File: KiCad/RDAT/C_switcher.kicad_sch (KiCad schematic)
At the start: 11 parts, among them J18 MUSBRM1C130, U10 CH224K

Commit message: Push before Board Layout
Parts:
- C78: footprint A_HDJ_Library:C_0402_1005Metric -> Capacitor_SMD:C_0402_1005Metric
- D126, D127, D128: footprint A_HDJ_Library:D_0402_1005Metric -> Diode_SMD:D_SOD-882
- J18: footprint A_HDJ_Library:USB_C_Receptacle_G-Switch_GT-USB-7010ASV -> footprints:AMPHENOL_MUSBRM1C130
- R69, R70, R71: footprint A_HDJ_Library:R_0402_1005Metric -> Resistor_SMD:R_0402_1005Metric
- U10: footprint A_HDJ_Library:ESSOP-10-1EP_3.9x5mm_P1.0mm_EP3.2x2.3 -> footprints:ESSOP-10_L4.9-W3.9-P1.0-LS6.0-TL-EP
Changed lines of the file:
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@@
+			"AAAAAAAAAAAAAAAAAAAAAAAAAAAAAAAAAAAAAAAAAAAAAAAAAAAAAAAAAAAAAAAAAAAAAAAAAAAA"
+			"AAAAAAAAAAAAAAAAAAAAAAAAAAAAAAAAAAAAAAAAAAAAAAAAAAAAAAAAAAAAAAAAAAAAAAAAAAAA"
+			"AAAAAAAAAAAAAAAAAAAAAAAAAAAAAAAAAAAAAAAAAAAAAAAAAAAAAAAAAAAAAAAAAAAAAAAAAAAA"
+			"AAAAAAAAAAAAAAAAAAAAAAAAAAAAAAAAAAAAAAAAAAAAAAAAAAAAAAAAAAAAAAAAAAAAAAAAAAAA"
+			"AAAAAAAAAAAAAAAAAAAAAAAAAAAAAAAAAAAAAAAAAAAAAAAAAAAAAAAAAAAAAAAAAAAAAAAAAAAA"
+			"AAAAAAAAAAAAAAAAAAAAAAAAAAAAAAAAAAAAAAAAAAAAAAAAAAAAAAAAAAAAAAAAAAAAAAAAAAAA"
+			"AAAAAAAAAAAAAAAAAAAAAAAAAAAAAAAAAAAAAAAAAAAAAAAAAAAAAAAAAAAAAAAAAAAAAAAAAAAA"
+			"AAAAAAAAAAAAAAAAAAAAAAAAAAAAAAAAAAAAAAAAAAAAAAAAAAAAAAAAAAAAAAAAAAAAAAAAAAAA"
+			"AAAAAAAAAAAAAAAAAAAAAAAAAAAAAAAAAAAAAAAAAAAAAAAAAAAAAAAAAAAAAAAAAAAAAAAAAAAA"
+			"AAAAAAAAAAAAAAAAAAAAAAAAAAAAAAAAAAAAAAAAAAAAAAAAAAAAAAAAAAAAAAAAAAAAAAAAAAAA"
+			"AAAAAAAAAAAAAAAAAAAAAAAAAAAAAAAAAAAAAAAAAAAAAAAAAAAAAAAAAAAAAAAAAAAAAAAAAAAA"
+			"AAAAAAAAAAAAAAAAAAAAAAAAAAAAAAAAAAAAAAAAAAAAAAAAAAAAAAAAAAAAAAAAAAAAAAAAAAAA"
+			"AAAAAAAAAAAAAAAAAAAAAAAAAAAAAAAAAAAAAAAAAAAAAAAAAAAAAAAAAAAAAAAAAAAAAAAAAAAA"
+			"AAAAAAAAAAAAAAAAAAAAAAAAAAAAAAAAAAAAAAAAAAAAAAAAAAAAAAAAAAAAAAAAAAAAAAAAAAAA"
+			"AAAAAAAAAAAAAAAAAAAAAAAAAAAAAAAAAAAAAAAAAAAAAAAAAAAAAAAAAAAAAAAAAAAAAAAAAAAA"
+			"AAAAAAAAAAAAAAAAAAAAAAAAAAAAAAAAAAAAAAAAAAAAAAAAAAAAAAAAAAAAAAAAAAAAAAAAAAAA"
+			"AAAAAAAAAAAAAAAAAAAAAAAAAAAAAAAAAAAAAAAAAAAAAAAAAAAAAAAAAAAAAAAAAAAAAAAAAAAA"
+			"AAAAAAAAAAAAAAAAAAAAAAAAAAAAAAAAAAAAAAAAAAAAAAAAAAAAAAAAAAAAAAAAAAAAAAAAAAAA"
 			"AAAAAAAAAAAAAAAAAAAAAAAAAAAAAAAAAAAAAAAAAAAAAAAAAAAAAAAAAAAAAAAAAAAAAAAAAAAA"
 			"AAAAAAAAAAAAAAAAAAAAAAAAAAAAAAAAAAAAAAAAAAAAAAAAAAAAAAAAAAAAAAAAAAAAAAAAAAAA"
@@
 			)
 		)
-		(property "Footprint" "A_HDJ_Library:USB_C_Receptacle_G-Switch_GT-USB-7010ASV"
+		(property "Footprint" "footprints:AMPHENOL_MUSBRM1C130"
 			(at 60.96 53.34 0)
 			(effects
@@
 			)
 		)
-		(property "Footprint" "A_HDJ_Library:ESSOP-10-1EP_3.9x5mm_P1.0mm_EP3.2x2.3"
+		(property "Footprint" "footprints:ESSOP-10_L4.9-W3.9-P1.0-LS6.0-TL-EP"
 			(at 149.86 48.26 0)
 			(effects
@@
 			)
 		)
-		(property "Footprint" "A_HDJ_Library:D_0402_1005Metric"
+		(property "Footprint" "Diode_SMD:D_SOD-882"
 			(at 109.22 66.04 0)
 			(effects
@@
 			)
 		)
-		(property "Footprint" "A_HDJ_Library:C_0402_1005Metric"
+		(property "Footprint" "Capacitor_SMD:C_0402_1005Metric"
 			(at 127 46.6852 0)
 			(effects
@@
 			)
 		)
-		(property "Footprint" "A_HDJ_Library:D_0402_1005Metric"
+		(property "Footprint" "Diode_SMD:D_SOD-882"
 			(at 116.84 66.04 0)
 			(effects
@@
 			)
 		)
-		(property "Footprint" "A_HDJ_Library:R_0402_1005Metric"
+		(property "Footprint" "Resistor_SMD:R_0402_1005Metric"
 			(at 129.794 37.084 90)
 			(effects
@@
 			)
 		)
-		(property "Footprint" "A_HDJ_Library:D_0402_1005Metric"
+		(property "Footprint" "Diode_SMD:D_SOD-882"
 			(at 101.6 66.04 0)
 			(effects
@@
 			)
 		)
-		(property "Footprint" "A_HDJ_Library:R_0402_1005Metric"
+		(property "Footprint" "Resistor_SMD:R_0402_1005Metric"
 			(at 174.244 42.164 90)
 			(effects
@@
 			)
 		)
-		(property "Footprint" "A_HDJ_Library:R_0402_1005Metric"
+		(property "Footprint" "Resistor_SMD:R_0402_1005Metric"
 			(at 129.794 40.894 90)
 			(effects

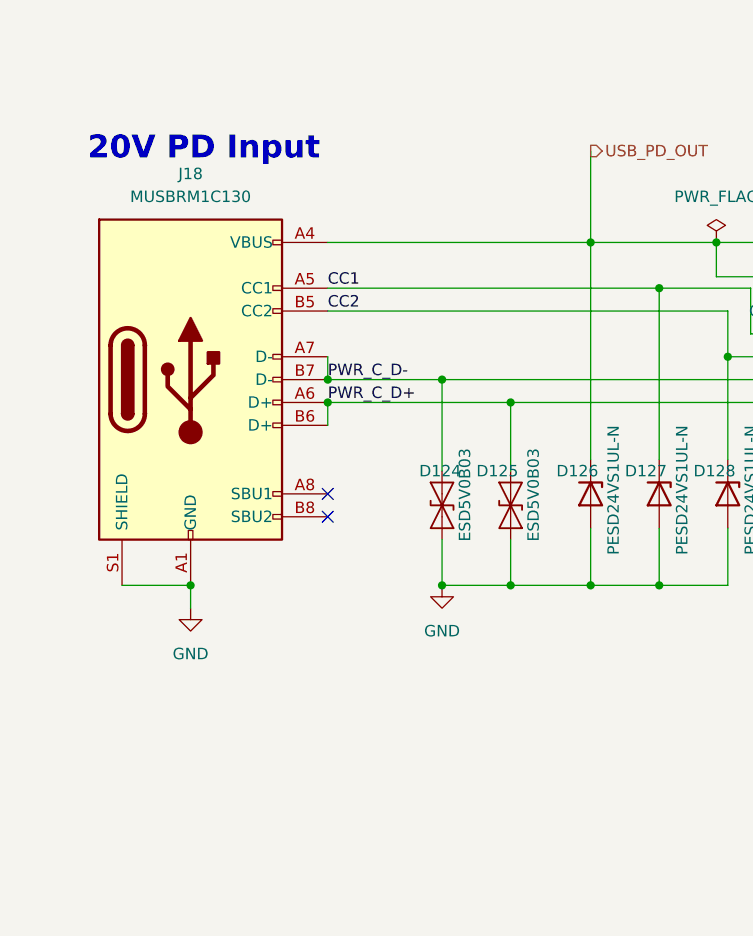
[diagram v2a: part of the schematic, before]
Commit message: Placed a lot of components
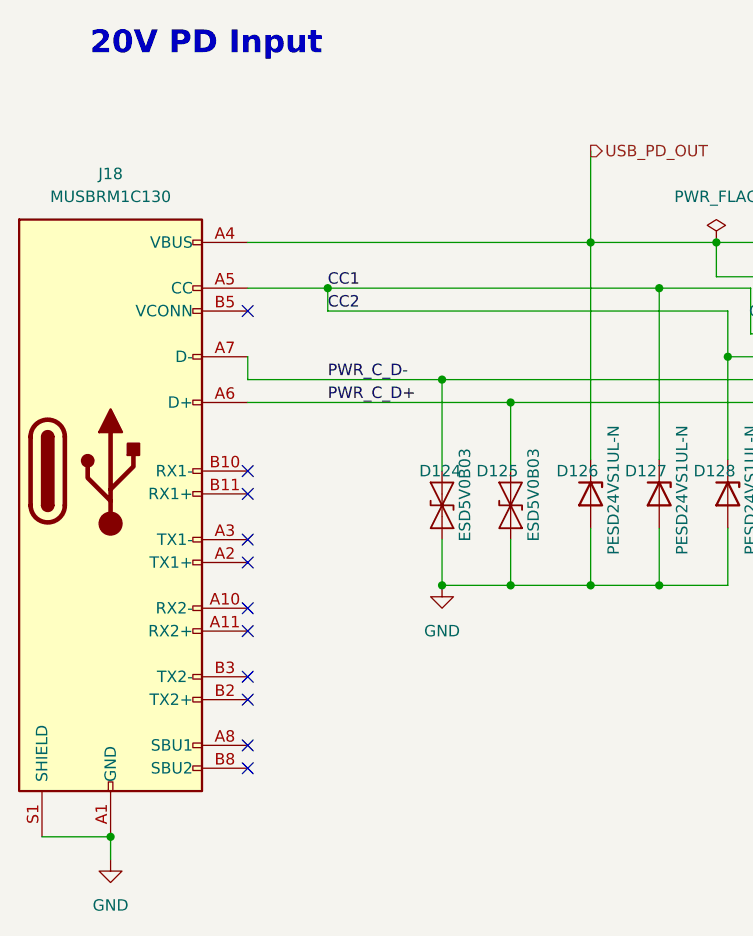
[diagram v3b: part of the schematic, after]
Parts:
- J18: symbol Connector:USB_C_Receptacle_USB2.0_16P -> Connector:USB_C_Plug
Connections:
- net CC1: now also D128.1 (K), U10.6 (CC2)
- net PWR_C_D+: no longer J18.B6 (D+)
- net PWR_C_D-: no longer J18.B7 (D-)
- removed net CC2: D128.1 (K), J18.B5 (CC2), U10.6 (CC2)
- no-connect marks 5 -> 14
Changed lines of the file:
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@@
 	(text "20V PD Input"
 		(exclude_from_sim no)
-		(at 45.72 29.21 0)
+		(at 45.974 17.526 0)
 		(effects
 			(font
@@
 	)
 	(junction
-		(at 72.39 53.34)
+		(at 72.39 43.18)
 		(diameter 0)
 		(color 0 0 0 0)
@@
 	)
 	(junction
-		(at 57.15 76.2)
-		(diameter 0)
-		(color 0 0 0 0)
-	)
-	(junction
-		(at 72.39 55.88)
-		(diameter 0)
-		(color 0 0 0 0)
-	)
-	(junction
 		(at 115.57 38.1)
 		(diameter 0)
@@
 		(color 0 0 0 0)
 	)
+	(junction
+		(at 48.26 104.14)
+		(diameter 0)
+		(color 0 0 0 0)
+	)
 	(no_connect
 		(at 162.56 45.72)
@@
 	)
 	(no_connect
-		(at 72.39 68.58)
+		(at 63.5 96.52)
 	)
 	(no_connect
-		(at 72.39 66.04)
+		(at 63.5 86.36)
+	)
+	(no_connect
+		(at 63.5 93.98)
+	)
+	(no_connect
+		(at 63.5 66.04)
+	)
+	(no_connect
+		(at 63.5 88.9)
+	)
+	(no_connect
+		(at 63.5 81.28)
 	)
 	(no_connect
 		(at 162.56 50.8)
 	)
+	(no_connect
+		(at 63.5 71.12)
+	)
+	(no_connect
+		(at 63.5 63.5)
+	)
+	(no_connect
+		(at 63.5 73.66)
+	)
+	(no_connect
+		(at 63.5 45.72)
+	)
+	(no_connect
+		(at 63.5 78.74)
+	)
 	(wire
 		(pts
@@
 	(wire
 		(pts
-			(xy 72.39 38.1) (xy 101.6 38.1)
-		)
-		(stroke
-			(width 0)
-			(type default)
-		)
-	)
-	(wire
-		(pts
 			(xy 139.7 38.1) (xy 139.7 43.18)
 		)
@@
 	(wire
 		(pts
-			(xy 49.53 76.2) (xy 57.15 76.2)
+			(xy 63.5 43.18) (xy 72.39 43.18)
+		)
+		(stroke
+			(width 0)
+			(type default)
+		)
+	)
+	(wire
+		(pts
+			(xy 40.64 104.14) (xy 48.26 104.14)
 		)
 		(stroke
@@
 	(wire
 		(pts
+			(xy 72.39 43.18) (xy 109.22 43.18)
+		)
+		(stroke
+			(width 0)
+			(type default)
+		)
+	)
+	(wire
+		(pts
 			(xy 101.6 38.1) (xy 101.6 62.23)
 		)
@@
 	(wire
 		(pts
+			(xy 72.39 43.18) (xy 72.39 45.72)
+		)
+		(stroke
+			(width 0)
+			(type default)
+		)
+	)
+	(wire
+		(pts
 			(xy 116.84 45.72) (xy 116.84 50.8)
 		)
@@
 	(wire
 		(pts
+			(xy 63.5 53.34) (xy 63.5 50.8)
+		)
+		(stroke
+			(width 0)
+			(type default)
+		)
+	)
+	(wire
+		(pts
 			(xy 137.16 45.72) (xy 134.62 45.72)
 		)
@@
 	(wire
 		(pts
-			(xy 57.15 76.2) (xy 57.15 78.74)
+			(xy 48.26 104.14) (xy 48.26 106.68)
+		)
+		(stroke
+			(width 0)
+			(type default)
+		)
+	)
+	(wire
+		(pts
+			(xy 63.5 53.34) (xy 85.09 53.34)
 		)
 		(stroke
@@
 	(wire
 		(pts
+			(xy 63.5 55.88) (xy 92.71 55.88)
+		)
+		(stroke
+			(width 0)
+			(type default)
+		)
+	)
+	(wire
+		(pts
 			(xy 116.84 50.8) (xy 116.84 62.23)
 		)
@@
 	(wire
 		(pts
-			(xy 72.39 43.18) (xy 109.22 43.18)
-		)
-		(stroke
-			(width 0)
-			(type default)
-		)
-	)
-	(wire
-		(pts
 			(xy 177.8 43.18) (xy 182.88 43.18)
 		)
@@
 	(wire
 		(pts
-			(xy 72.39 53.34) (xy 85.09 53.34)
-		)
-		(stroke
-			(width 0)
-			(type default)
-		)
-	)
-	(wire
-		(pts
 			(xy 137.16 41.91) (xy 133.35 41.91)
 		)
@@
 	(wire
 		(pts
-			(xy 72.39 50.8) (xy 72.39 53.34)
-		)
-		(stroke
-			(width 0)
-			(type default)
-		)
-	)
-	(wire
-		(pts
 			(xy 92.71 76.2) (xy 85.09 76.2)
 		)
@@
 	(wire
 		(pts
-			(xy 72.39 55.88) (xy 72.39 58.42)
+			(xy 63.5 38.1) (xy 101.6 38.1)
 		)
 		(stroke
@@
 		(pts
 			(xy 125.73 41.91) (xy 115.57 41.91)
-		)
-		(stroke
-			(width 0)
-			(type default)
-		)
-	)
-	(wire
-		(pts
-			(xy 72.39 55.88) (xy 92.71 55.88)
 		)
 		(stroke
@@
 			"AAAAAAAAAAAAAAAAAAAAAAAAAAAAAAAAAAAAAAAAAAAAAAAAAAAAAAAAAAAAAAAAAAAAAAAAAAAA"
 			"AAAAAAAAAAAAAAAAAAAAAAAAAAAAAAAAAAAAAAAAAAAAAAAAAAAAAAAAAAAAAAAAAAAAAAAAAAAA"
-			"AAAAAAAAAAAAAAAAAAAAAAAAAAAAAAAAAAAAAAAAAAAAAAAAAA=="
+			"AAAAAAAAAAAAAAAAAAAAAAAAAAAAAAAAAAAAAAAAAAAAAAAAAAAAAAAAAAAAAAAAAAAAAAAAAAAA"
+			"AAAAAAAAAAAAAAAAAAAAAAAAAAAAAAAAAAAAAAAAAAAAAAAAAAAAAAAAAAAAAAAAAAAAAAAAAAAA"
+			"AAAAAAAAAAAAAAAAAAAAAAAAAAAAAAAAAAAAAAAAAAAAAAAAAAAAAAAAAAAAAAAAAAAAAAAAAAAA"
+			"AAAAAAAAAAAAAAAAAAAAAAAAAAAAAAAAAAAAAAAAAAAAAAAAAAAAAAAAAAAAAAAAAAAAAAAAAAAA"
+			"AAAAAAAAAAAAAAAAAAAAAAAAAAAAAAAAAAAAAAAAAAAAAAAAAAAAAAAAAAAAAAAAAAAAAAAAAAAA"
+			"AAAAAAAAAAAAAAAAAAAAAAAAAAAAAAAAAAAAAAAAAAAAAAAAAAAAAAAAAAAAAAAAAAAAAAAAAAAA"
+			"AAAAAAAAAAAAAAAAAAAAAAAAAAAAAAAAAAAAAAAAAAAAAAAAAAAAAAAAAAAAAAAAAAAAAAAAAAAA"
+			"AAAAAAAAAAAAAAAAAAAAAAAAAAAAAAAAAAAAAAAAAAAAAAAAAAAAAAAAAAAAAAAAAAAAAAAAAAAA"
+			"AAAAAAAAAAAAAAAAAAAAAAAAAAAAAAAAAAAAAAAAAAAAAAAAAAAAAAAAAAAAAAAAAAAAAAAAAAAA"
+			"AAAAAAAAAAAAAAAAAAAAAAAAAAAAAAAAAAAAAAAAAAAAAAAAAAAAAAAAAAAAAAAAAAAAAAAAAAAA"
+			"AAAAAAAAAAAAAAAAAAAAAAAAAAAAAAAAAAAAAAAAAAAAAAAAAAAAAAAAAAAAAAAAAAAAAAAAAAAA"
+			"AAAAAAAAAAAAAAAAAAAAAAAAAAAAAAAAAAAAAAAAAAAAAAAAAAAAAAAAAAAAAAAAAAAAAAAAAAAA"
+			"AAAAAAAAAAAAAAAAAAAAAAAAAAAAAAAAAAAAAAAAAAAAAAAAAAAAAAAAAAAAAAAAAAAAAAAAAAAA"
+			"AAAAAAAAAAAAAAAAAAAAAAAAAAAAAAAAAAAAAAAAAAAAAAAAAAAAAAAAAAAAAAAAAAAAAAAAAAAA"
+			"AAAAAAAAAAAAAAAAAAAAAAAAAAAAAAAAAAAAAAAAAAAAAAAAAAAAAAAAAAAAAAAAAAAAAAAAAAAA"
+			"AAAAAAAAAAAAAAAAAAAAAAAAAAAAAAAAAAAAAAAAAAAAAAAAAAAAAAAAAAAAAAAAAAAAAAAAAAAA"
+			"AAAAAAAAAAAAAAAAAAAAAAAAAAAAAAAAAAAAAAAAAAAAAAAAAAAAAAAAAAAAAAAAAAAAAAAAAAAA"
+			"AAAAAAAAAAAAAAAAAAAAAAAAAAAAAAAAAAAAAAAAAAAAAAAAAAAAAAAAAAAAAAAAAAAAAAAAAAAA"
+			"AAAAAAAAAAAAAAAAAAAAAAAAAAAAAAAAAAAAAAAAAAAAAAAAADxaasFS9p7GP+ygQQAAAAAACJ7A"
+			"pGrqbmUca8FETxerveOgQQAAAAAACJ7AYD09B/Hea8G2AgmBN9ugQQAAAAAACJ7ALKg0s9+hbMFi"
+			"unVFrdKgQQAAAAAACJ7AAACwoDFlbcEAIF/1HsqgQQAAAAAACJ7A1JmO/eYobsFK3caNjMGgQQAA"
+			"AAAACJ7AoMqv9//sbsH6m64L9rigQQAAAAAACJ7AXOfyvHyxb8HIBRhsW7CgQQAAAAAACJ7AgKKb"
+			"vS47cMFuxASsvKegQQAAAAAACJ7AQhwuMNGdcMGmgXbIGZ+gQQAAAAAACJ7AcIsgzaUAccEo526+"
+			"cpagQQAAAAAACJ7Ahppiq6xjccGunu+Kx42gQQAAAAAACJ7AAPTj4eXGccHwUfoqGIWgQQAAAAAA"
+			"CJ7AWkKUh1EqcsGqqpCbZHygQQAAAAAACJ7AEDBjs++NcsGSUrTZrHOgQQAAAAAACJ7AnmdAfMDx"
+			"csFk82bi8GqgQQAAAAAACJ7AgJMb+cNVc8HaNqqyMGKgQQAAAAAACJ7AMl7kQPq5c8Grxn9HbFmg"
+			"QQAAAAAACJ7AMHKKamMedMGQTOmdo1CgQQAAAAAACJ7A9nn9jP+CdMFEcuiy1kegQQAAAAAACJ7A"
+			"ACAtv87ndMGA4X6DBT+gQQAAAAAACJ7Ayg4JGNFMdcH9Q64MMDagQQAAAAAACJ7A0PCArgaydcF0"
+			"Q3hLVi2gQQAAAAAACJ7AgDgD8At9dsE2wOLdlRugQQAAAAAACJ7A8EoxO99Id8GSpcsixAmgQQAA"
+			"AAAACJ7AAHyIR4EVeMGggoAEwu+fQQAAAAAACJ7AkB+GzPLieMF6wpvI2MufQQAAAAAACJ7AgImn"
+			"gTSxecFEpgNizKefQQAAAAAACJ7AsA1qHkeAesGUydKgnIOfQQAAAAAACJ7AAABLWitQe8EAyCNV"
+			"SV+fQQAAAAAACJ7AULTH7OEgfMEcPRFP0jqfQQAAAAAACJ7AgH5djWvyfMF8xLVeNxafQQAAAAAA"
+			"CJ7AcLKJ88jEfcG2+StUePGeQQAAAAAACJ7AAKTJ1vqXfsFgeI7/lMyeQQAAAAAACJ7AEKea7gFs"
+			"f8EO3PcwjaeeQQAAAAAACJ7AwAc9eW8ggMFUwIK4YIKeQQAAAAAACJ7AmJjyTEmLgMHIwElmD12e"
+			"QQAAAAAACJ7AALAszo72gMEAeWcKmTeeQQAAAAAACJ7A6PepWEBigcGQhPZ0/RGeQQAAAAAACJ7A"
+			"QBopSF7OgcEMfxF2POydQQAAAAAACJ7AAJYnxeCngsEgr1V8SaCdQQAAAAAACJ7AwHIdIxmDg8Hk"
+			"5QievlOdQQAAAAAACJ7AAAAAQApghMEAAABcmgadQQAAAAAACA=="
 		)
 	)
@@
 	)
 	(symbol
-		(lib_id "Connector:USB_C_Receptacle_USB2.0_16P")
-		(at 57.15 53.34 0)
+		(lib_id "Connector:USB_C_Plug")
+		(at 48.26 63.5 0)
 		(unit 1)
 		(exclude_from_sim no)
@@
 		(fields_autoplaced yes)
 		(property "Reference" "J18"
-			(at 57.15 30.48 0)
+			(at 48.26 30.48 0)
 			(effects
 				(font
@@
 		)
 		(property "Value" "MUSBRM1C130"
-			(at 57.15 33.02 0)
+			(at 48.26 33.02 0)
 			(effects
 				(font
@@
 		)
 		(property "Footprint" "footprints:AMPHENOL_MUSBRM1C130"
-			(at 60.96 53.34 0)
+			(at 52.07 63.5 0)
 			(effects
 				(font
@@
 			)
 		)
-		(property "Datasheet" "https://cdn.amphenol-cs.com/media/wysiwyg/files/documentation/datasheet/inputoutput/io_harsh_musb-type-c.pdf"
-			(at 60.96 53.34 0)
+		(property "Datasheet" "https://www.usb.org/sites/default/files/documents/usb_type-c.zip"
+			(at 52.07 63.5 0)
 			(effects
 				(font
@@
 			)
 		)
-		(property "Description" ""
-			(at 57.15 53.34 0)
+		(property "Description" "USB Type-C Plug connector"
+			(at 48.26 63.5 0)
 			(effects
 				(font
@@
 		)
 		(property "SCH_Show_Footprint" ""
-			(at 57.15 53.34 0)
+			(at 48.26 63.5 0)
 			(effects
 				(font
@@
 		)
 		(property "Sim.Device" ""
-			(at 57.15 53.34 0)
+			(at 48.26 63.5 0)
 			(effects
 				(font
@@
 		)
 		(property "Sim.Pins" ""
-			(at 57.15 53.34 0)
+			(at 48.26 63.5 0)
 			(effects
 				(font
@@
 		)
 		(property "Sim.Type" ""
-			(at 57.15 53.34 0)
+			(at 48.26 63.5 0)
 			(effects
 				(font
@@
 		)
 		(property "JLCPCB_LINK" "https://www.digikey.com/en/products/detail/amphenol-cs-commercial-products/MUSBRM1C130/5877551"
-			(at 57.15 53.34 0)
+			(at 48.26 63.5 0)
 			(effects
 				(font
@@
 		(pin "B8"
 		)
-		(pin "B6"
+		(pin "B10"
 		)
 		(pin "A8"
@@
 		(pin "B9"
 		)
-		(pin "B7"
+		(pin "A10"
 		)
 		(pin "A9"
 		)
 		(pin "A1"
+		)
+		(pin "A11"
+		)
+		(pin "A3"
+		)
+		(pin "B3"
+		)
+		(pin "A2"
+		)
+		(pin "B2"
+		)
+		(pin "B11"
 		)
 		(instances
@@
 	(symbol
 		(lib_id "power:GND")
-		(at 57.15 78.74 0)
+		(at 48.26 106.68 0)
 		(unit 1)
 		(exclude_from_sim no)
@@
 		(fields_autoplaced yes)
 		(property "Reference" "#PWR079"
-			(at 57.15 85.09 0)
+			(at 48.26 113.03 0)
 			(effects
 				(font
@@
 		)
 		(property "Value" "GND"
-			(at 57.15 83.82 0)
+			(at 48.26 111.76 0)
 			(effects
 				(font
@@
 		)
 		(property "Footprint" ""
-			(at 57.15 78.74 0)
+			(at 48.26 106.68 0)
 			(effects
 				(font
@@
 		)
 		(property "Datasheet" ""
-			(at 57.15 78.74 0)
+			(at 48.26 106.68 0)
 			(effects
 				(font
@@
 		)
 		(property "Description" ""
-			(at 57.15 78.74 0)
+			(at 48.26 106.68 0)
 			(effects
 				(font

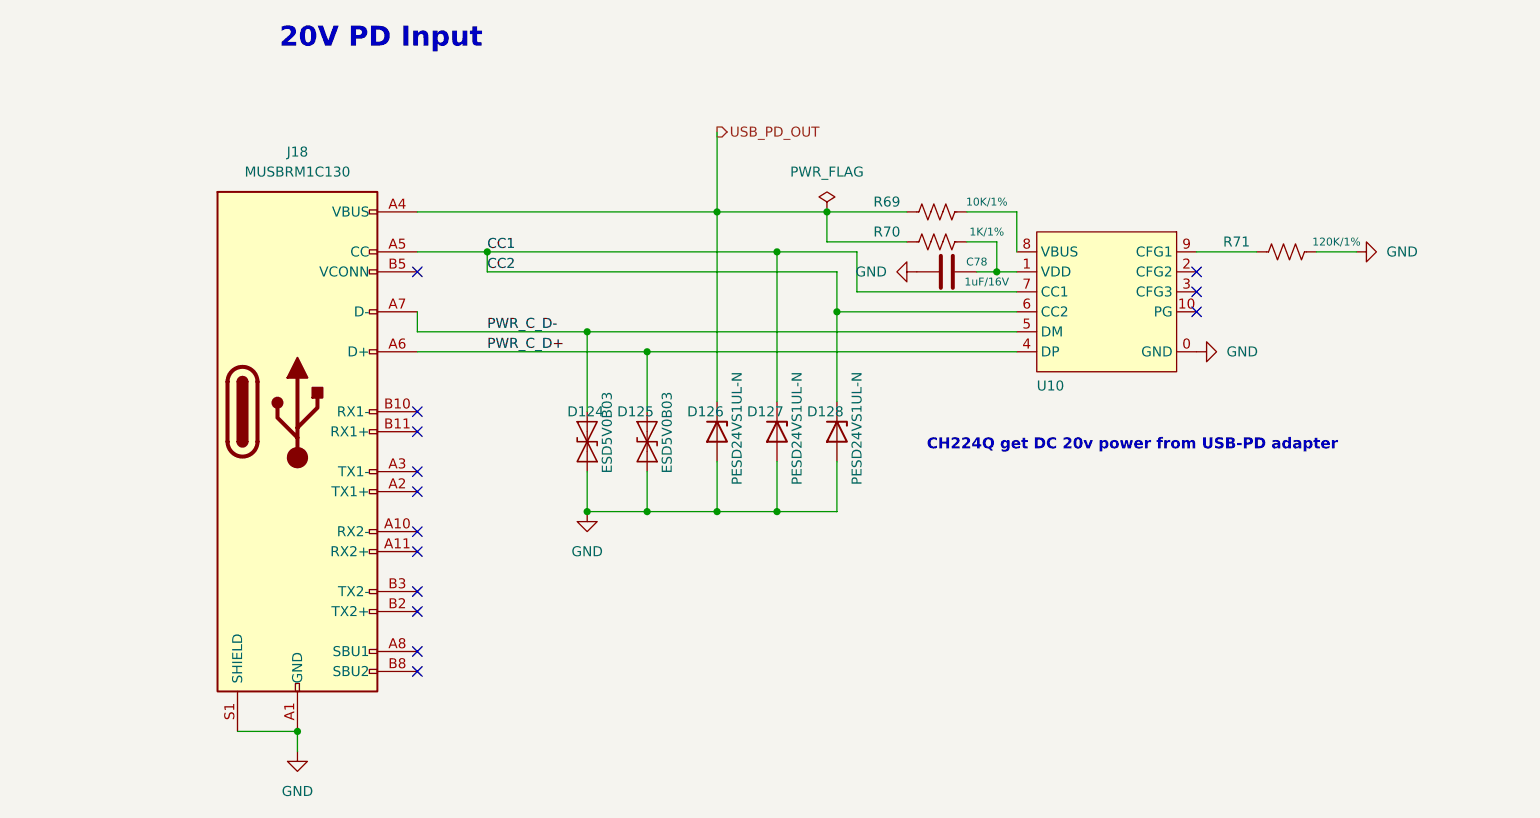
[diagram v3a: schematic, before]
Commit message: End Of day commit
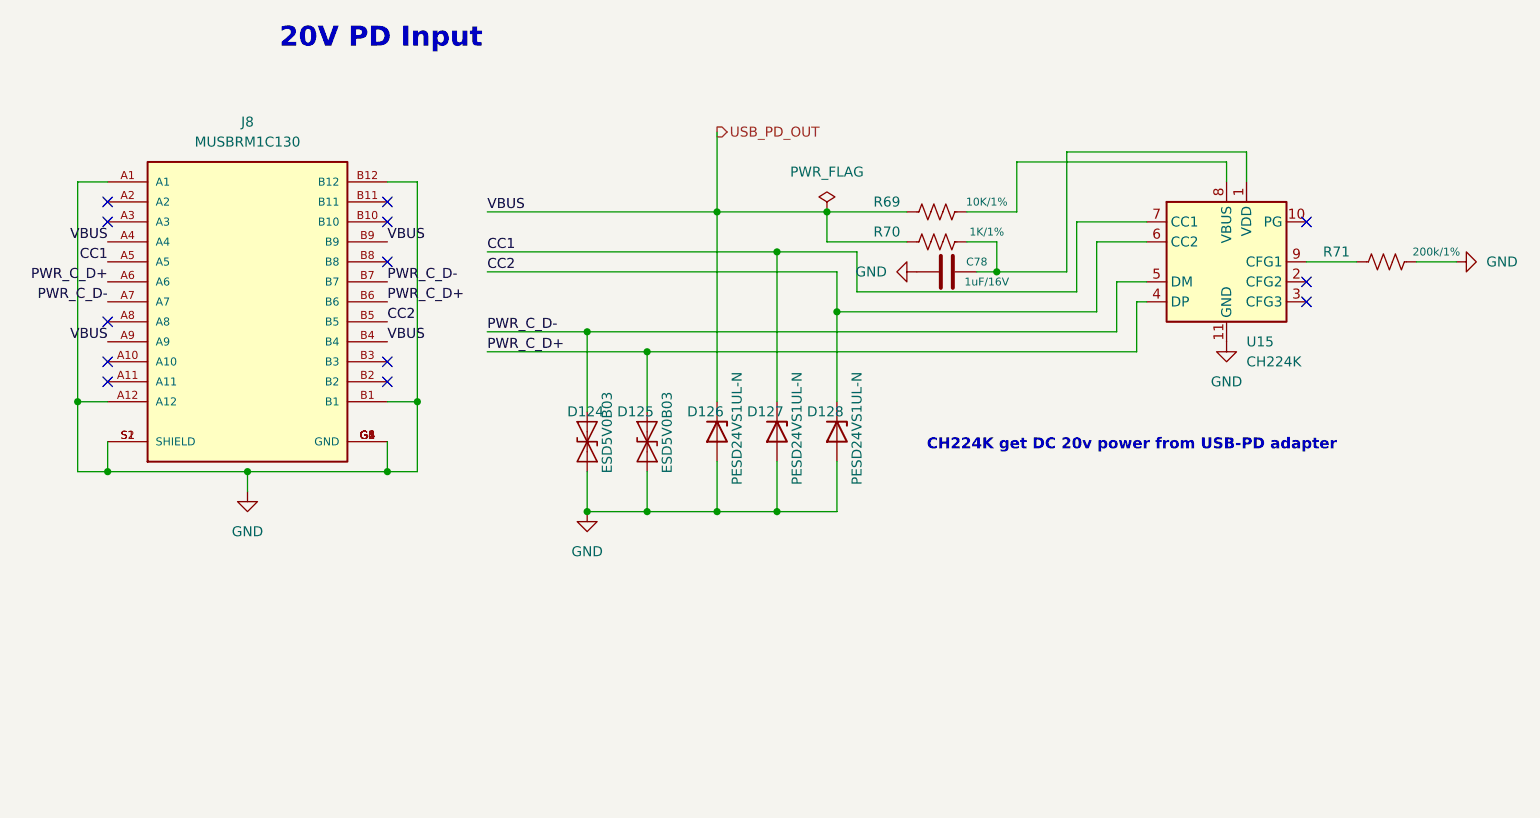
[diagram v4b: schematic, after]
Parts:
- removed J18: MUSBRM1C130, footprints:AMPHENOL_MUSBRM1C130, symbol Connector:USB_C_Plug
- removed U10: CH224K, footprints:ESSOP-10_L4.9-W3.9-P1.0-LS6.0-TL-EP, symbol A_HDJ_Library:CH224K
- added J8: MUSBRM1C130, footprints:AMPHENOL_MUSBRM1C130, symbol MUSBRM1C130:MUSBRM1C130
- added U15: CH224K, Package_SO:SSOP-10-1EP_3.9x4.9mm_P1mm_EP2.1x3.3mm, symbol Interface_USB:CH224K
- R71: value 120K/1% -> 200k/1%; JLCPCB_LINK https://jlcpcb.com/partdetail/26493-0402WGF1203TCE/C25750 -> (none)
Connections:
- net CC1: now also J8.A5, U15.7 (CC1); no longer D128.1 (K)
- net GND: now also J8.A1, J8.A12, J8.B1, J8.B12, J8.G1 (GND), J8.G2 (GND), J8.G3 (GND), J8.G4 (GND), J8.G5 (GND), J8.G6 (GND), J8.S1 (SHIELD), J8.S2 (SHIELD), U15.11 (GND)
- net PWR_C_D+: now also J8.A6, J8.B6, U15.4 (DP)
- net PWR_C_D-: now also J8.A7, J8.B7, U15.5 (DM)
- net USB_PD_OUT: now also J8.A4, J8.A9, J8.B4, J8.B9
- net at C78.1, R70.2: now also U15.1 (VDD)
- net at R69.2: now also U15.8 (VBUS)
- net at R71.1: now also U15.9 (CFG1)
- new net CC2: D128.1 (K), J8.B5, U15.6 (CC2)
- no-connect marks 14 -> 13
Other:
- note added: "CH224K get DC 20v power from USB-PD adapter"
- note removed: "CH224Q get DC 20v power from USB-PD adapter"
- moved on the sheet: R71
